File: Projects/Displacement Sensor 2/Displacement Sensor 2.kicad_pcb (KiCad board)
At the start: 2 copper layers, 16 parts, among them J1 DTF13-6P, U1 TJA1050DRG, U2 MCP2515-I, X1 8MHz

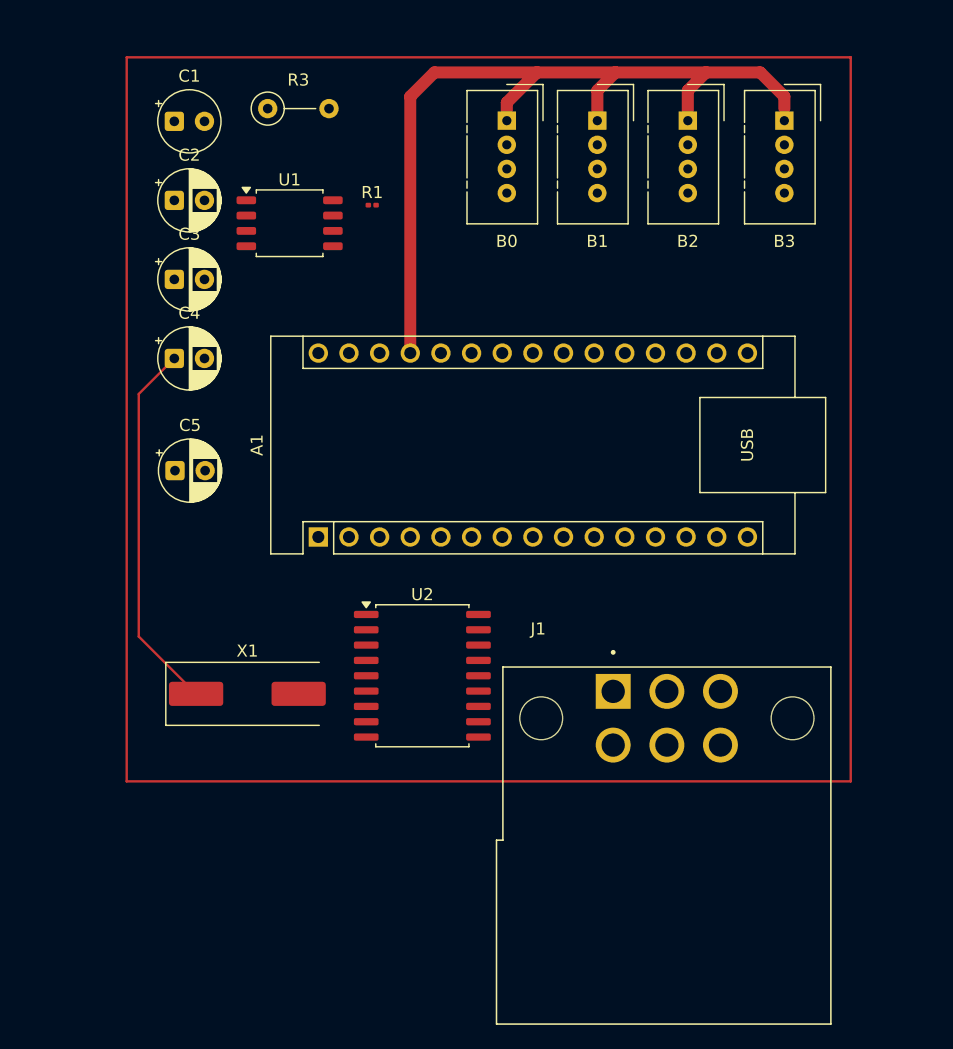
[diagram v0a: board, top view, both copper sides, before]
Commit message: PCB Draft 1
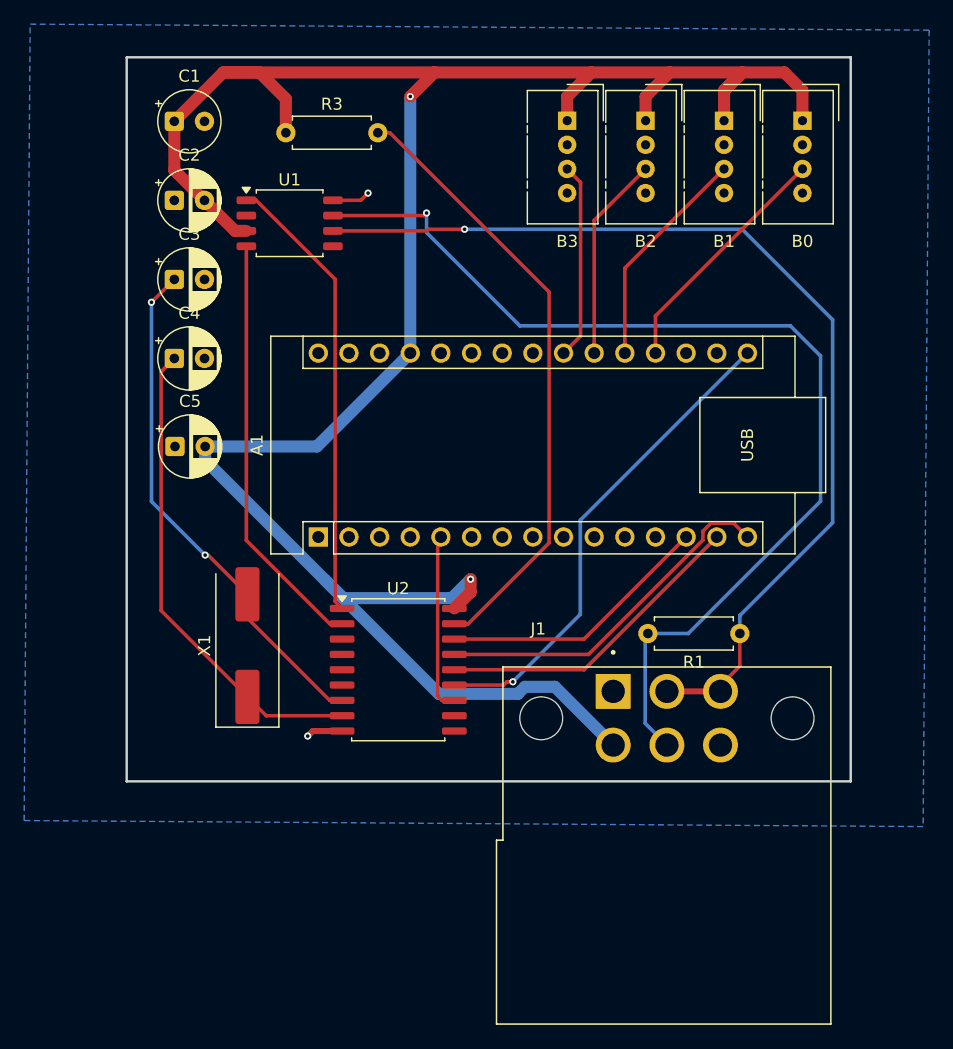
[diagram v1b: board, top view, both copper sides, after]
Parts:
- R1: value 120k -> 120; footprint Resistor_SMD:R_0201_0603Metric -> Resistor_THT:R_Axial_DIN0207_L6.3mm_D2.5mm_P7.62mm_Horizontal
- R3: footprint Resistor_THT:R_Axial_DIN0207_L6.3mm_D2.5mm_P5.08mm_Vertical -> Resistor_THT:R_Axial_DIN0207_L6.3mm_D2.5mm_P7.62mm_Horizontal
- moved R1 46.8 mm to (167.3, 97.0), turned to 180 degrees
- moved B0 24.5 mm to (172.5, 54.5)
- moved B3 18.0 mm to (153.0, 54.5)
- moved B1 10.5 mm to (166.0, 54.5)
- moved X1 4.00 mm to (126.5, 98.0), turned to 90 degrees
- moved B2 3.50 mm to (159.5, 54.5)
- moved R3 2.50 mm to (129.7, 55.5)
- moved U2 2.06 mm to (139.0, 100.0)
- moved C5 2.00 mm to (120.5, 81.5)
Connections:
- C1 pad 2: 0 -> GND
- C2 pad 1: 0 -> GND
- C3 pad 2: 0 -> GND
- C4 pad 2: 0 -> GND
- C5 pad 1: 0 -> GND
- R1 pad 1: High -> Low
- R1 pad 2: Low -> High
- U1 pad 2: 0 -> GND
- U1 pad 8: 0 -> GND
- U2 pad 9: 0 -> GND
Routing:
- net +5V: track 69.2 -> 200.2 mm, vias 0 -> 2
- net High: track 0.00 -> 87.3 mm, vias 0 -> 1
- net Low: track 0.00 -> 83.8 mm, vias 0 -> 1
- net Net-(U2-~{RESET}): track 0.00 -> 51.1 mm
- net Net-(U2-OSC2): track 0.00 -> 43.0 mm, vias 0 -> 2
- net SCK: track 0.00 -> 40.3 mm, vias 0 -> 1
- net Net-(U1-TXD): track 0.00 -> 37.6 mm
- net Net-(U1-RXD): track 0.00 -> 35.2 mm
- net SO: track 0.00 -> 29.7 mm
- net SI: track 0.00 -> 26.3 mm
- net CS: track 0.00 -> 22.7 mm
- net Net-(A1-A0): track 0.00 -> 20.3 mm
- net Net-(A1-A1): track 0.00 -> 18.7 mm
- net Net-(A1-A2): track 0.00 -> 17.0 mm
- net Net-(A1-A3): track 0.00 -> 16.9 mm
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- added copper zone on B.Cu, net GND
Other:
- board outline added: 60 x 60 mm
